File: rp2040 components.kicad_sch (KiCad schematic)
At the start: 29 parts, among them J1 SWD, J2 USB_C_Receptacle_USB2.0, SW27 SW_Push, U2 W25Q128JVS, U3 XC6206PxxxMR, U4 USBLC6-2SC6, Y1 12MHz

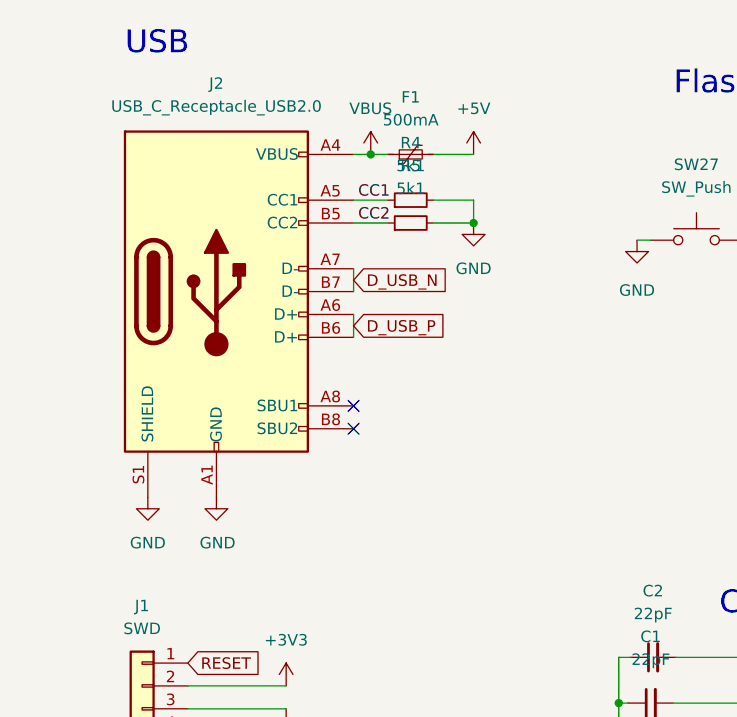
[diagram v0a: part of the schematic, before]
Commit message: galvy edits - start routing testing
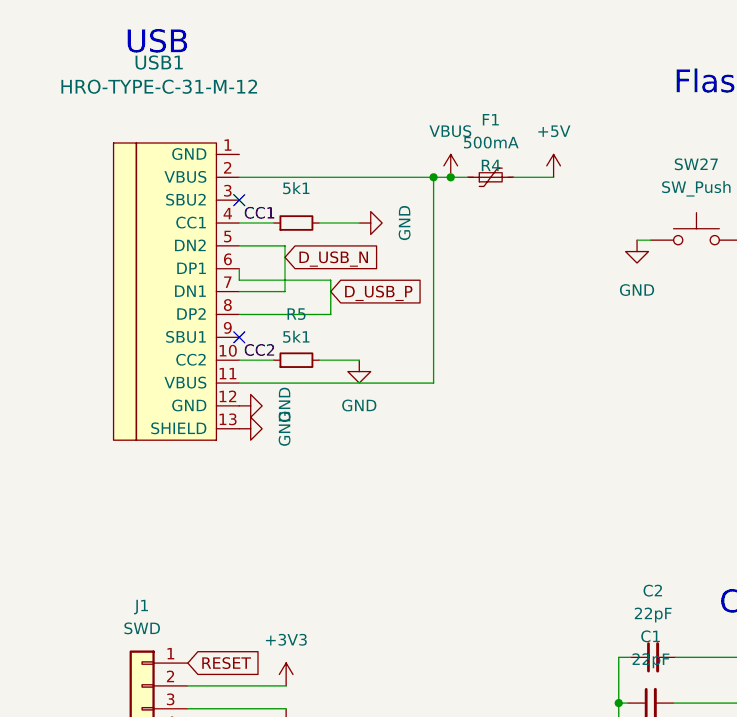
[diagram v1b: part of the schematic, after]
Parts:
- removed J2: USB_C_Receptacle_USB2.0, Connector_USB:USB_C_Receptacle_HRO_TYPE-C-31-M-12, symbol Connector:USB_C_Receptacle_USB2.0
- added USB1: HRO-TYPE-C-31-M-12, Type-C:HRO-TYPE-C-31-M-12-HandSoldering, symbol Type-C:HRO-TYPE-C-31-M-12
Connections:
- net CC1: now also USB1.4 (CC1)
- net CC2: now also USB1.10 (CC2)
- net D_USB_N: now also USB1.5 (DN2), USB1.7 (DN1)
- net D_USB_P: now also USB1.6 (DP1), USB1.8 (DP2)
- net GND: now also USB1.12 (GND), USB1.13 (SHIELD)
- net VBUS: now also USB1.11 (VBUS), USB1.2 (VBUS)
